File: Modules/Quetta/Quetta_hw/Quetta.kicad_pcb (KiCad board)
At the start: 2 copper layers, 89.6 x 37 mm, 89 parts, among them Q1 IRLML9303, SW1 SWITCH_H

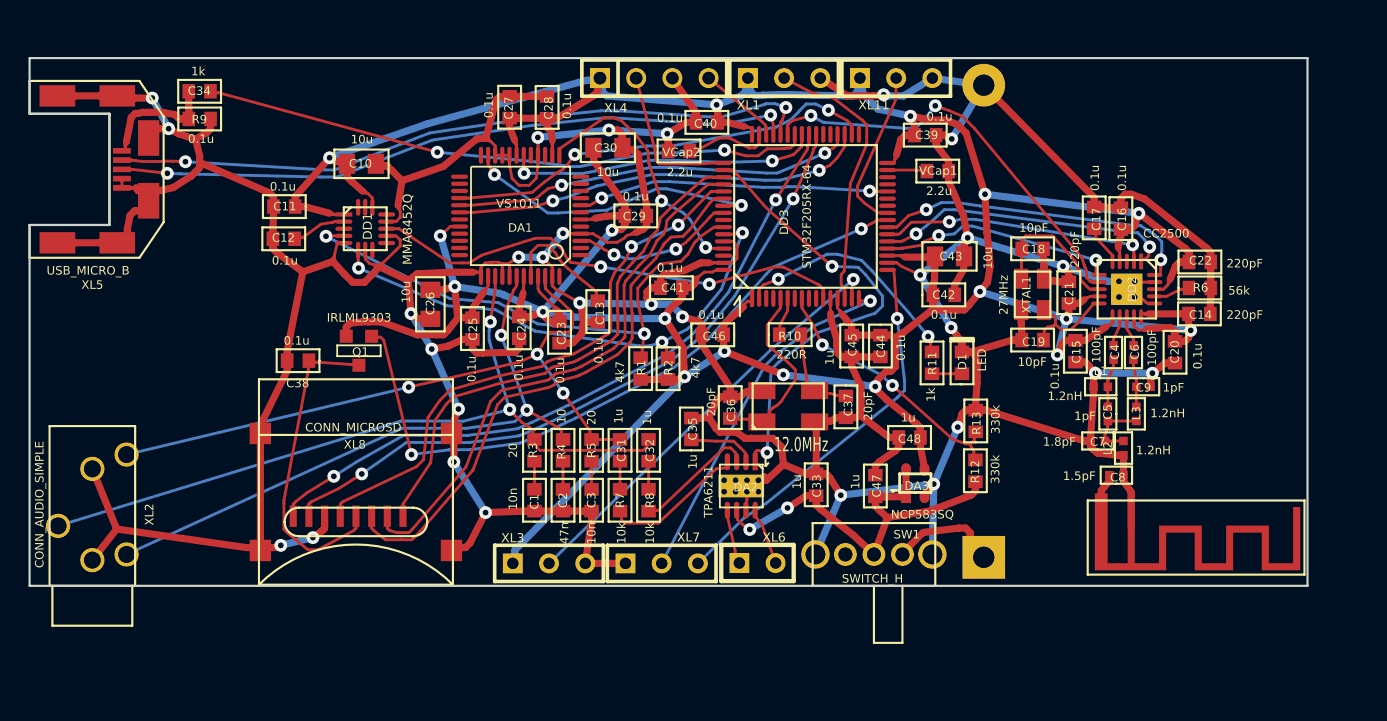
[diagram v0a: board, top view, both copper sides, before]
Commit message: + Quetta Gerber + Quetta Portrait, speaking
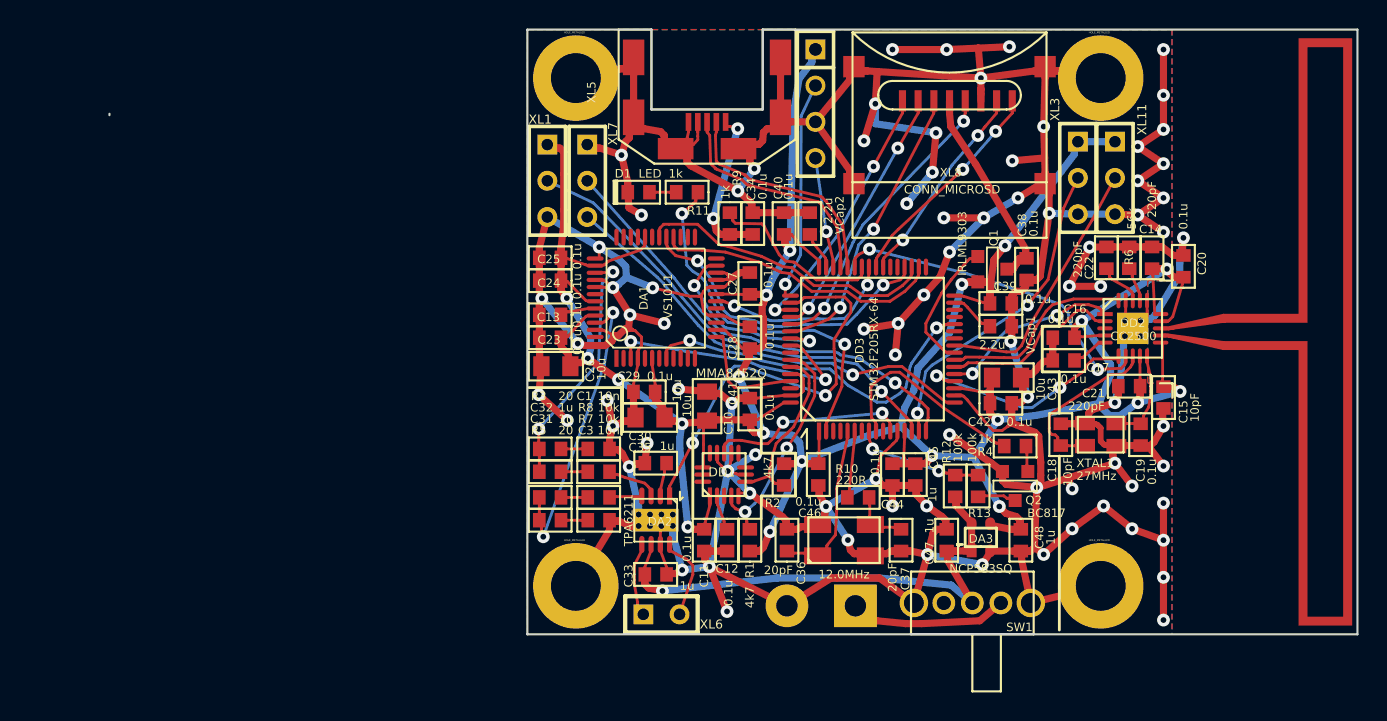
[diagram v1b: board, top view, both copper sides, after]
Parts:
- removed C2: 47n, CAP_0603
- removed C4, C6: 100pF, CAP_0402
- removed C5, C9: 1pF, CAP_0402
- removed C7: 1.8pF, CAP_0402
- removed C8: 1.5pF, CAP_0402
- removed L1, L2, L3: 1.2nH, IND_0402
- removed XL2: CONN_AUDIO_SIMPLE, CONN_AUDIO_CKX3_5_30
- added HOLE1: HOLE_METALLED, Hole3_5_out6mm, F.Cu at (187.4, 104.4)
- added HOLE2: HOLE_METALLED, Hole3_5_out6mm, F.Cu at (187.4, 140.0)
- added HOLE3: HOLE_METALLED, Hole3_5_out6mm, F.Cu at (224.2, 104.4)
- added HOLE4: HOLE_METALLED, Hole3_5_out6mm, F.Cu at (224.2, 140.0)
- added Q2: BC817, SOT23, F.Cu at (218.2, 133.0)
- ANT1: value ANT_GENERAL -> ANT_PCB_NOCNTR; footprint ANT_2400_MEANDER -> ANT_FOLDED_DIPOLE2
- R12, R13: value 330k -> 100k
- R4: value 10 -> 1k
- moved C38 51.5 mm to (219.0, 117.8), turned to 270 degrees
- moved XL8 48.2 mm to (213.6, 108.4), turned to 90 degrees
- moved XL3 45.9 mm to (222.6, 111.4), turned to 270 degrees
- moved Q1 44.8 mm to (216.6, 117.8), turned to 90 degrees
- moved XL5 42.1 mm to (196.6, 106.6), turned to 270 degrees
- moved C34 39.5 mm to (199.8, 114.6), turned to 90 degrees
- moved XL10 39.0 mm to (202.2, 141.4)
- moved R9 38.3 mm to (198.2, 114.6), turned to 270 degrees
- moved C11 37.6 mm to (196.4, 136.8), turned to 270 degrees
- moved C12 37.6 mm to (198.0, 136.8), turned to 270 degrees
- moved R4 31.7 mm to (218.2, 130.2), turned to 0 degrees
- moved DD1 30.5 mm to (197.8, 132.2), turned to 0 degrees
- moved C10 29.6 mm to (196.6, 127.4), turned to 90 degrees
- moved XL7 27.3 mm to (188.2, 111.6), turned to 270 degrees
- moved D1 25.6 mm to (191.8, 112.4), turned to 180 degrees
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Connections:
- ANT1 pad 1: GND -> /Ant1
- ANT1 pad 2: GND -> /Ant2
- C22 pad 1: +3.3V -> N-0000023
- DA1 pad 42: /SND_C -> (no net)
- DD2 pad 18: +3.3V -> N-0000023
- DD3 pad 9: (no net) -> /BAT_MEASURE
- R13 pad 2: GND -> N-0000045
- R4 pad 1: N-0000046 -> /BAT_MEASURE
- R4 pad 2: /SND_C -> N-0000046
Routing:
- net +3.3V: track 318.4 -> 244.8 mm, vias 18 -> 20
- net /SND_C: track 43.7 -> 0.00 mm, vias 2 -> 0
- net /SD_POWER: track 47.5 -> 9.32 mm, vias 2 -> 0
- net /SND_R: track 54.3 -> 17.2 mm
- net GND: track 467.4 -> 502.0 mm, vias 29 -> 83
- net /SD_DAT0: track 48.0 -> 14.4 mm
- net /USB_DM: track 49.3 -> 16.1 mm, vias 2 -> 0
- net /SD_DAT1: track 48.4 -> 15.5 mm
- net /USB_DP: track 47.5 -> 16.1 mm, vias 2 -> 0
- net N-0000055: track 42.7 -> 12.3 mm, vias 2 -> 0
- net /SND_L: track 46.8 -> 20.8 mm, vias 3 -> 2
- net /I2C_SDA: track 36.0 -> 12.4 mm, vias 3 -> 0
- net /I2C_SCL: track 37.8 -> 16.2 mm
- net /SD_DAT3: track 38.3 -> 18.0 mm, vias 0 -> 2
- net /ACC_IRQ: track 33.9 -> 14.1 mm
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- added copper zone on B.Cu, net GND
- added copper zone on F.Cu, net GND
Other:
- board size 89.6 x 37 mm -> 87.5 x 42.4 mm
- rule pad_to_mask_clearance: 0.2 -> 0.075
